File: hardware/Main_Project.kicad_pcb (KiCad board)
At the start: 2 copper layers, 87 x 87.6 mm, 2 parts

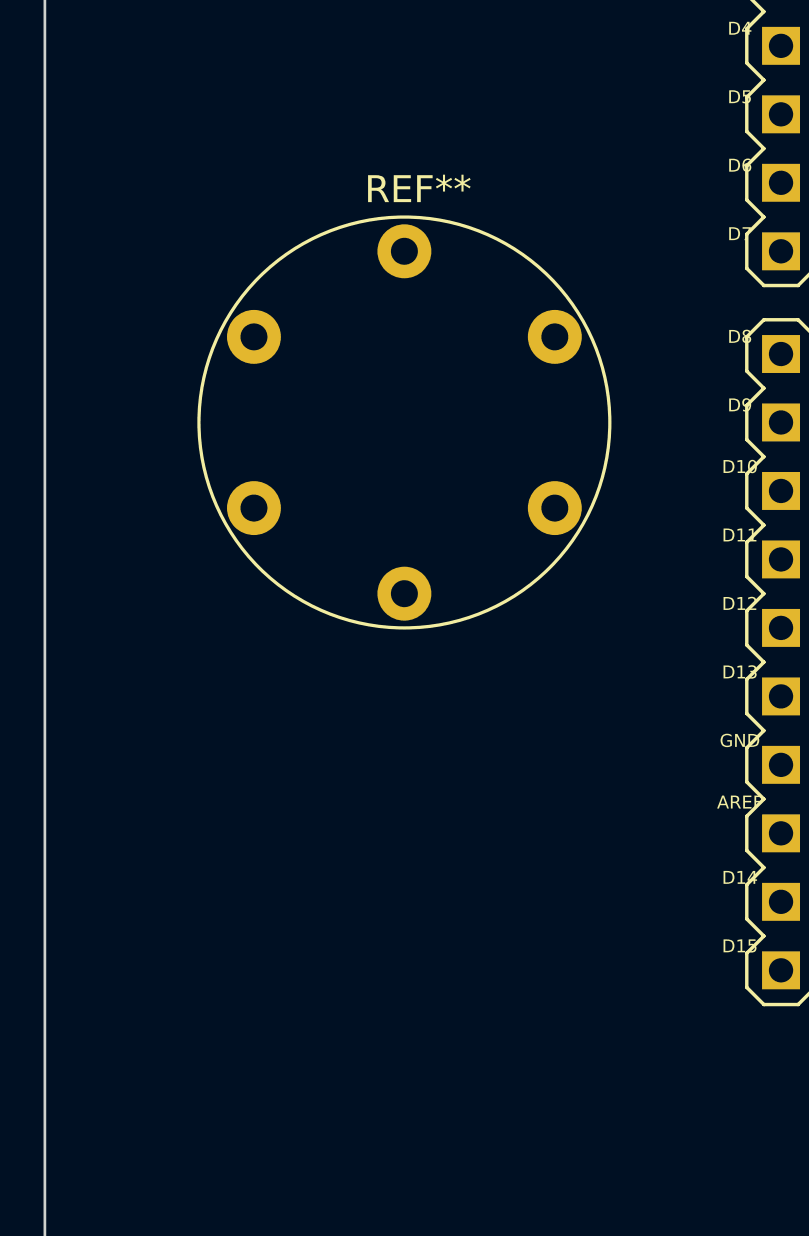
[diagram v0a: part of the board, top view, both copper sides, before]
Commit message: Minor changes
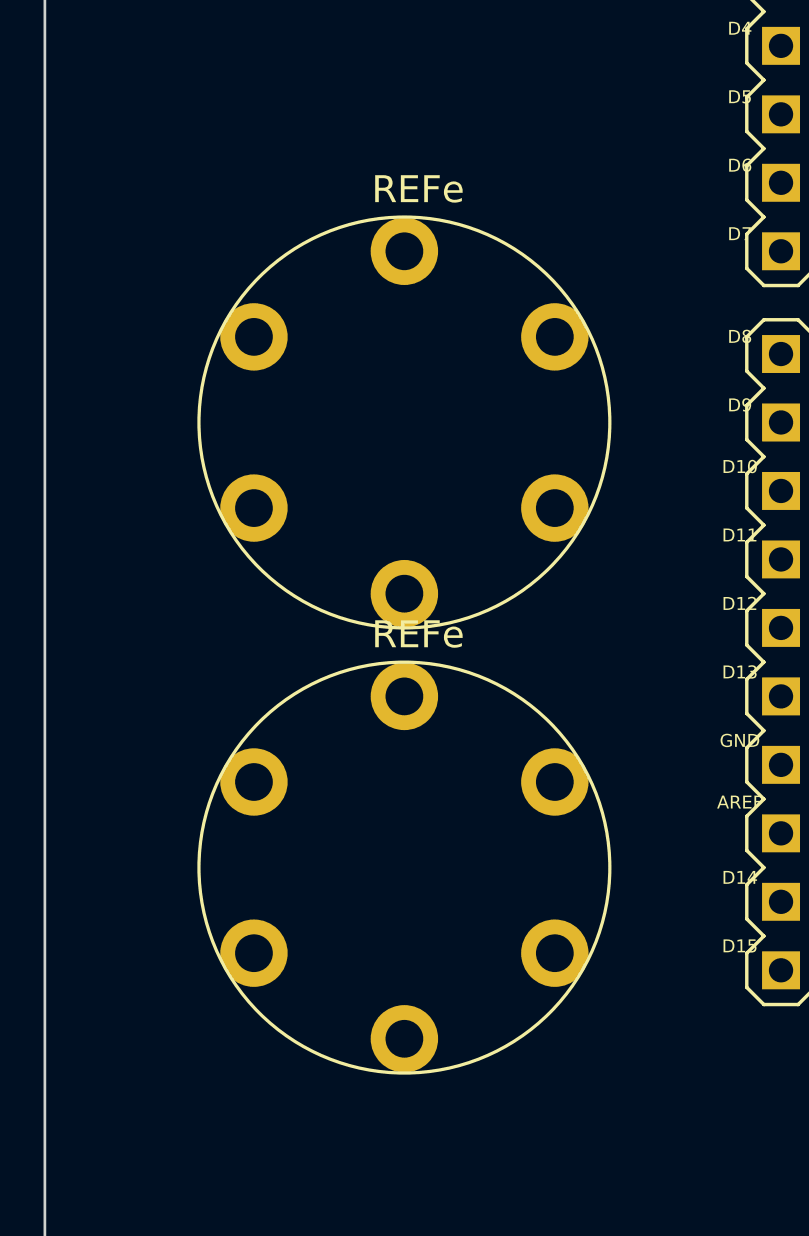
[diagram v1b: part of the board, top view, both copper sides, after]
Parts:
- added REFe: Adafruit_Flora_Sensor, TDP3KICAD:Adafruit_Flora_Sensor, F.Cu at (165.1, 106.7)
- renumbered REF** to REFe
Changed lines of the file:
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@@
   )
   (net 0 "")
+  (footprint "TDP3KICAD:Adafruit_Flora_Sensor" (layer "F.Cu")
+    (at 165.1 106.68)
+    (attr through_hole)
+    (fp_text reference "REFe" (at 0.508 -8.636 unlocked) (layer "F.SilkS")
+        (effects (font (size 1 1) (thickness 0.15)))
+    )
+    (fp_text value "Adafruit_Flora_Sensor" (at 0.254 -10.16 unlocked) (layer "F.Fab")
+        (effects (font (size 1 1) (thickness 0.15)))
+    )
+    (fp_circle (center 0 0) (end 7.62 0)
+      (stroke (width 0.12) (type default)) (fill none) (layer "F.SilkS"))
+    (pad "1" thru_hole circle (at 0 -6.35) (size 2.5 2.5) (drill 1.4) (layers "*.Cu" "*.Mask"))
+    (pad "2" thru_hole circle (at -5.58 -3.175) (size 2.5 2.5) (drill 1.4) (layers "*.Cu" "*.Mask"))
+    (pad "3" thru_hole circle (at -5.58 3.175) (size 2.5 2.5) (drill 1.4) (layers "*.Cu" "*.Mask"))
+    (pad "4" thru_hole circle (at 0 6.35) (size 2.5 2.5) (drill 1.4) (layers "*.Cu" "*.Mask"))
+    (pad "5" thru_hole circle (at 5.58 3.175) (size 2.5 2.5) (drill 1.4) (layers "*.Cu" "*.Mask"))
+    (pad "6" thru_hole circle (at 5.58 -3.175) (size 2.5 2.5) (drill 1.4) (layers "*.Cu" "*.Mask"))
+    (model ":MYLIBRARIESMOD:TDP3.pretty/Adafruit Flora TCS34725.step" hide
+      (offset (xyz -148.5 105 3.5))
+      (scale (xyz 1 1 1))
+      (rotate (xyz 0 0 0))
+    )
+    (model ":MYLIBRARIESMOD:TDP3.pretty/flora uv sensor v6.step"
+      (offset (xyz 0 0 0))
+      (scale (xyz 0.87 0.87 0.9))
+      (rotate (xyz 0 0 90))
+    )
+  )
   (footprint "TDP3KICAD:FRDM_KL25Z_NORMAL" (layer "F.Cu")
     (at 203.2 83.82)
@@
     (fp_line (start 26.4 -29.2) (end 26.4 37)
       (stroke (width 0.127) (type solid)) (layer "F.Fab"))
-    (fp_arc (start -26.4 -28.8) (mid -24.069771 -34.727634) (end -18.2 -37.2)
-      (stroke (width 0.127) (type solid)) (layer "F.Fab"))
-    (fp_arc (start -18 45.4) (mid -23.927634 43.069771) (end -26.4 37.2)
-      (stroke (width 0.127) (type solid)) (layer "F.Fab"))
-    (fp_arc (start 18 -37.2) (mid 23.927634 -34.869771) (end 26.4 -29)
-      (stroke (width 0.127) (type solid)) (layer "F.Fab"))
-    (fp_arc (start 26.4 37) (mid 24.069771 42.927634) (end 18.2 45.4)
+    (fp_arc (start -26.4 -28.8) (mid -24.069771 -34.727633) (end -18.2 -37.2)
+      (stroke (width 0.127) (type solid)) (layer "F.Fab"))
+    (fp_arc (start -18 45.4) (mid -23.927633 43.069771) (end -26.4 37.2)
+      (stroke (width 0.127) (type solid)) (layer "F.Fab"))
+    (fp_arc (start 18 -37.2) (mid 23.927633 -34.869771) (end 26.4 -29)
+      (stroke (width 0.127) (type solid)) (layer "F.Fab"))
+    (fp_arc (start 26.4 37) (mid 24.069771 42.927633) (end 18.2 45.4)
       (stroke (width 0.127) (type solid)) (layer "F.Fab"))
     (pad "3V3" thru_hole rect (at 24.13 15.24) (size 1.408 1.408) (drill 0.9) (layers "*.Cu" "*.Mask")
@@
     (at 165.1 90.17)
     (attr through_hole)
-    (fp_text reference "REF**" (at 0.508 -8.636 unlocked) (layer "F.SilkS")
+    (fp_text reference "REFe" (at 0.508 -8.636 unlocked) (layer "F.SilkS")
         (effects (font (size 1 1) (thickness 0.15)))
     )
@@
     (fp_circle (center 0 0) (end 7.62 0)
       (stroke (width 0.12) (type default)) (fill none) (layer "F.SilkS"))
-    (pad "1" thru_hole circle (at 0 -6.35) (size 2 2) (drill 1) (layers "*.Cu" "*.Mask"))
-    (pad "2" thru_hole circle (at -5.58 -3.175) (size 2 2) (drill 1) (layers "*.Cu" "*.Mask"))
-    (pad "3" thru_hole circle (at -5.58 3.175) (size 2 2) (drill 1) (layers "*.Cu" "*.Mask"))
-    (pad "4" thru_hole circle (at 0 6.35) (size 2 2) (drill 1) (layers "*.Cu" "*.Mask"))
-    (pad "5" thru_hole circle (at 5.58 3.175) (size 2 2) (drill 1) (layers "*.Cu" "*.Mask"))
-    (pad "6" thru_hole circle (at 5.58 -3.175) (size 2 2) (drill 1) (layers "*.Cu" "*.Mask"))
+    (pad "1" thru_hole circle (at 0 -6.35) (size 2.5 2.5) (drill 1.4) (layers "*.Cu" "*.Mask"))
+    (pad "2" thru_hole circle (at -5.58 -3.175) (size 2.5 2.5) (drill 1.4) (layers "*.Cu" "*.Mask"))
+    (pad "3" thru_hole circle (at -5.58 3.175) (size 2.5 2.5) (drill 1.4) (layers "*.Cu" "*.Mask"))
+    (pad "4" thru_hole circle (at 0 6.35) (size 2.5 2.5) (drill 1.4) (layers "*.Cu" "*.Mask"))
+    (pad "5" thru_hole circle (at 5.58 3.175) (size 2.5 2.5) (drill 1.4) (layers "*.Cu" "*.Mask"))
+    (pad "6" thru_hole circle (at 5.58 -3.175) (size 2.5 2.5) (drill 1.4) (layers "*.Cu" "*.Mask"))
+    (model ":MYLIBRARIESMOD:TDP3.pretty/Adafruit Flora TCS34725.step" hide
+      (offset (xyz -148.5 105 3.5))
+      (scale (xyz 1 1 1))
+      (rotate (xyz 0 0 0))
+    )
+    (model ":MYLIBRARIESMOD:TDP3.pretty/flora uv sensor v6.step"
+      (offset (xyz 0 0 0))
+      (scale (xyz 0.87 0.87 0.9))
+      (rotate (xyz 0 0 90))
+    )
   )
   (gr_rect (start 151.765 44.45) (end 238.76 132.08)
